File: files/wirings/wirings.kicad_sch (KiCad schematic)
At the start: 6 parts

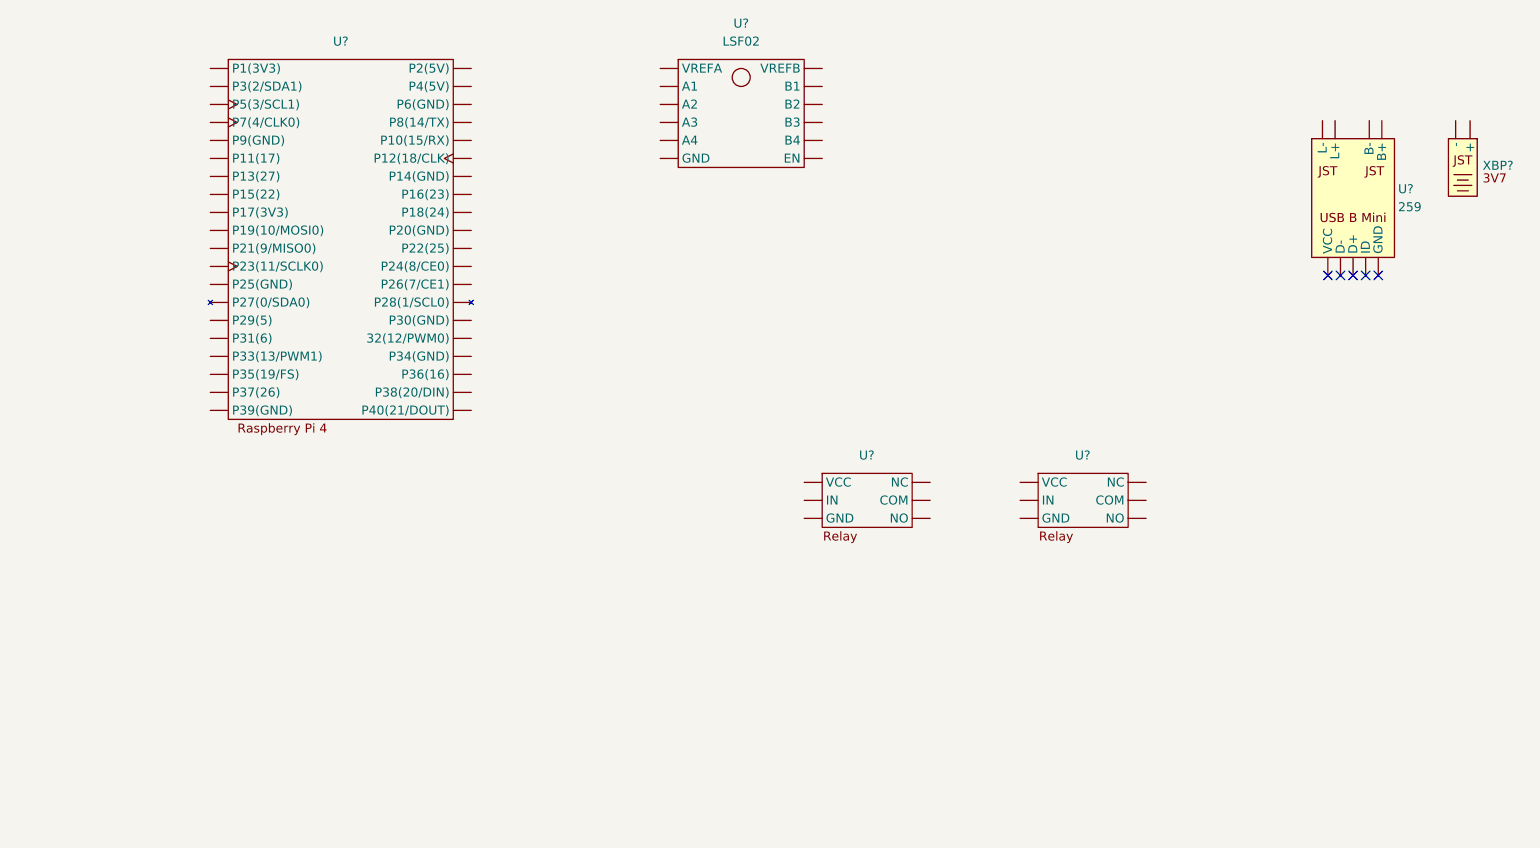
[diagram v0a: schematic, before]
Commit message: 14062023
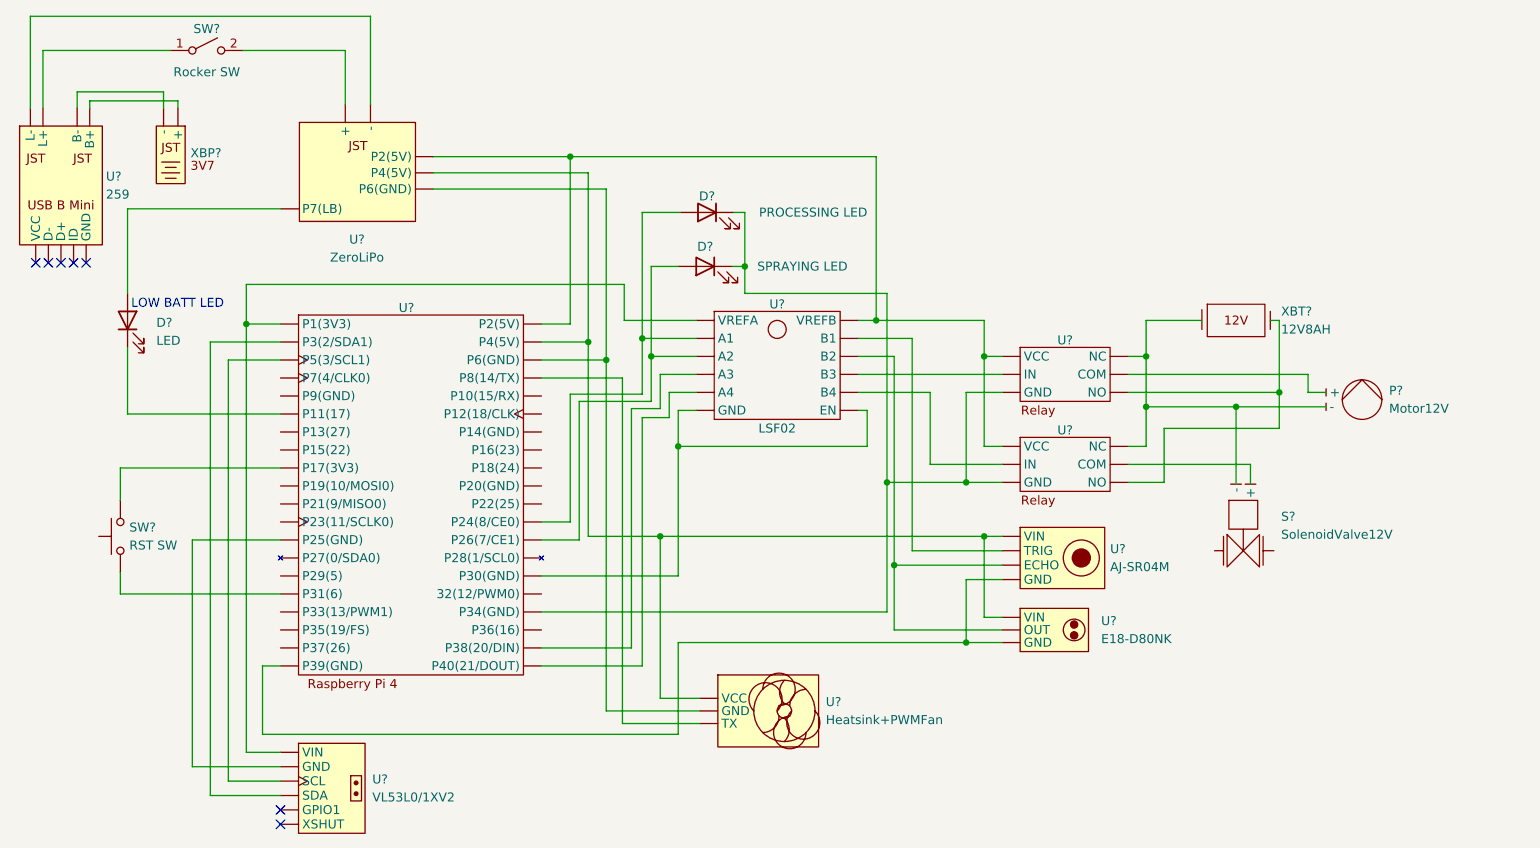
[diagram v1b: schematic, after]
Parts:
- added D?: PROCESSING LED, symbol Device:LED
- added D?: SPRAYING LED, symbol Device:LED
- added D?: LED, symbol Device:LED
- added P?: Motor12V, symbol Sensors and Others:Motor12V
- added S?: SolenoidValve12V, symbol Sensors and Others:SolenoidValve12V
- added SW?: Rocker SW, symbol Switch:SW_SPST
- added SW?: RST SW, symbol Switch:SW_Push
- added U?: VL53L0/1XV2, symbol Sensors and Others:VL53L0/1XV2
- added U?: Heatsink+PWMFan, symbol Sensors and Others:Heatsink+PWMFan
- added U?: E18-D80NK, symbol Sensors and Others:E18-D80NK
- added U?: ZeroLiPo, symbol Battery Power and Management:ZeroLiPo
- added U?: AJ-SR04M, symbol Sensors and Others:AJ-SR04M
- added XBT?: 12V8AH, symbol Battery Power and Management:12V8AH
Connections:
- net at U?. (VCC): now also P?. (-)
- net at U?. (VCC): now also U?. (VREFB)
- net at U?. (VCC): now also U?. (P7(LB))
- net at U?. (P9(GND)): now also D?.1 (K)
- net at XBP?. (-): now also U?. (VCC)
- net at U?. (VREFB): now also U?. (VIN)
- new net: P?. (-), S?. (-), U?. (VCC), U?. (VCC), XBT?. (-)
- new net: U?. (P7(LB)), U?. (P9(GND)), U?. (VCC), U?. (VCC), U?. (VREFB)
- new net: D?.1 (K), D?.1 (K), U?. (P9(GND)), U?. (VCC), U?. (VCC)
- new net: U?. (VCC), U?. (VCC), XBT?. (-)
- new net: U?. (VCC), U?. (VREFB)
- new net: S?. (-), U?. (VCC)
- new net: U?. (P9(GND)), U?. (XSHUT) (x3)
- new net: U?. (P9(GND)), U?. (VREFB), U?. (XSHUT)
- new net: U?. (P9(GND)), U?. (VCC)
- new net: U?. (P7(LB)), U?. (P9(GND)), U?. (VCC), U?. (VIN), U?. (VIN)
- new net: U?. (P7(LB)), U?. (P9(GND)), U?. (VCC)
- new net: U?. (VCC), XBP?. (-)
- new net: SW?.1 (A), U?. (VCC)
- new net: U?. (P9(GND)), U?. (VREFB) (x3)
- new net: D?.2 (A), U?. (P9(GND)), U?. (VREFB) (x2)
- new net: SW?.1, U?. (P9(GND))
- new net: SW?.2, U?. (P9(GND))
- new net: U?. (P9(GND)), U?. (VIN), U?. (VIN)
- new net: SW?.2 (B), U?. (P7(LB))
- new net: U?. (VIN), U?. (VIN), U?. (VREFB)
- new net: D?.2 (A), U?. (P7(LB))
- no-connect marks 5 -> 7
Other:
- note added: "LOW BATT LED"
- company: (none) -> There Goes Mangoes
- title: (none) -> Map of Wirings
- moved on the sheet: U?, XBP?

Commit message: 21062023
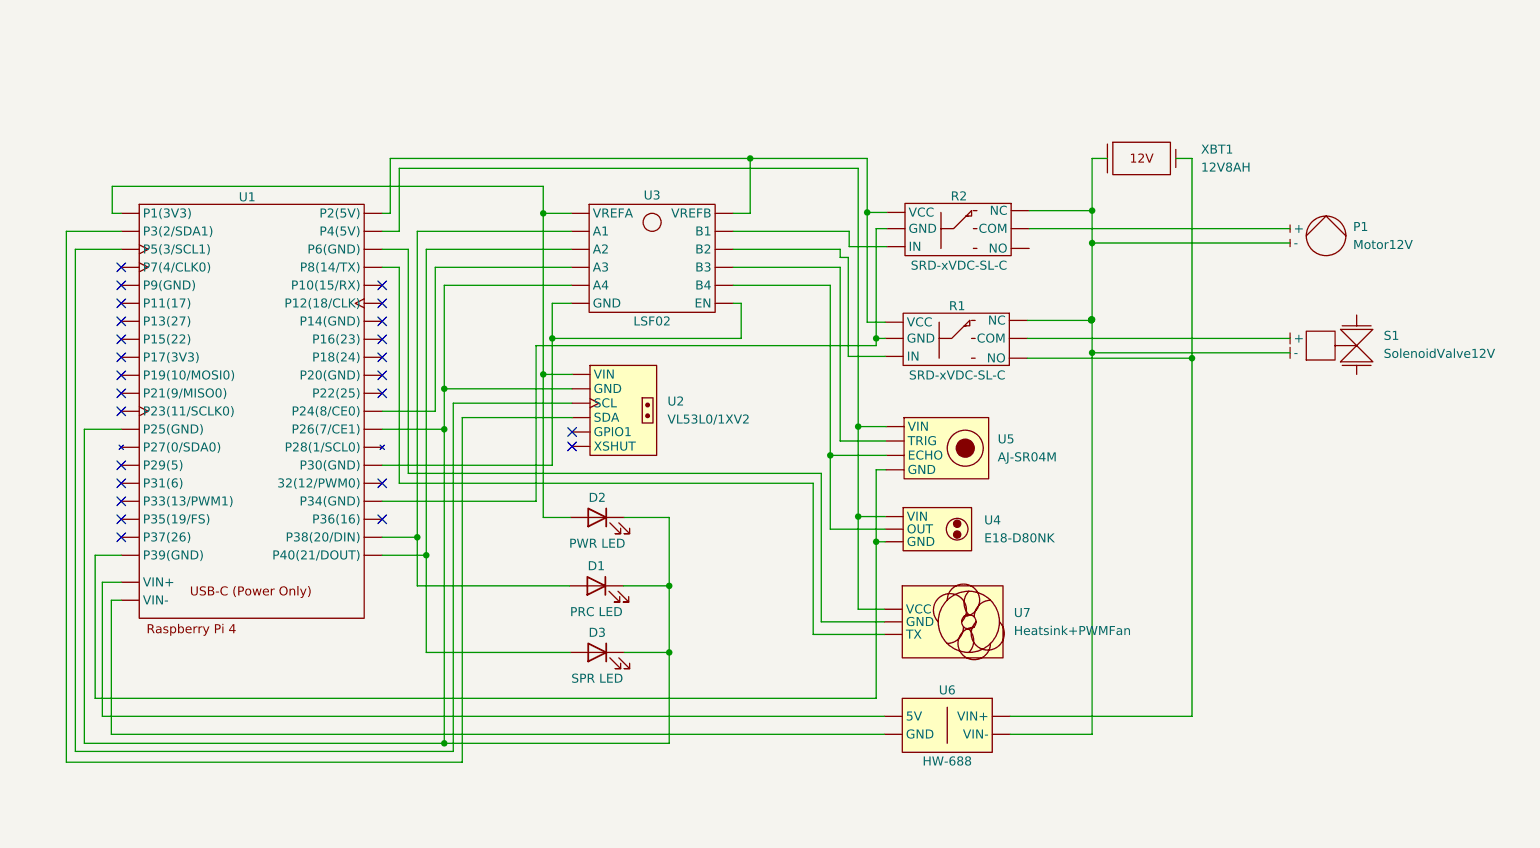
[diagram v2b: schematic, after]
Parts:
- removed D?: PROCESSING LED, symbol Device:LED
- removed D?: SPRAYING LED, symbol Device:LED
- removed D?: LED, symbol Device:LED
- removed P?: Motor12V, symbol Sensors and Others:Motor12V
- removed S?: SolenoidValve12V, symbol Sensors and Others:SolenoidValve12V
- removed SW?: Rocker SW, symbol Switch:SW_SPST
- removed SW?: RST SW, symbol Switch:SW_Push
- removed U? (x2): Songle_SRD-xxVDC-SL-C, symbol Relay:Songle_SRD-xxVDC-SL-C
- removed U?: VL53L0/1XV2, symbol Sensors and Others:VL53L0/1XV2
- removed U?: Heatsink+PWMFan, symbol Sensors and Others:Heatsink+PWMFan
- removed U?: 259, symbol Battery Power and Management:259
- removed U?: RPi4_Objective, symbol Raspberry Pi 4:RPi4_Objective
- removed U?: LSF02, symbol Multilevel Voltage Converter:LSF02
- removed U?: E18-D80NK, symbol Sensors and Others:E18-D80NK
- removed U?: ZeroLiPo, symbol Battery Power and Management:ZeroLiPo
- removed U?: AJ-SR04M, symbol Sensors and Others:AJ-SR04M
- removed XBP?: ICR18650-JST2P-PACK, symbol Battery Power and Management:ICR18650-JST2P-PACK
- removed XBT?: 12V8AH, symbol Battery Power and Management:12V8AH
- added D1: PRC LED, symbol Device:LED
- added D2: PWR LED, symbol Device:LED
- added D3: SPR LED, symbol Device:LED
- added P1: Motor12V, symbol Sensors and Others:Motor12V
- added R1, R2: SRD-xVDC-SL-C, symbol Sensors and Others:SRD-xVDC-SL-C
- added S1: SolenoidValve12V, symbol Sensors and Others:SolenoidValve12V
- added U1: RPi4_Objective, symbol Raspberry Pi 4:RPi4_Objective
- added U2: VL53L0/1XV2, symbol Sensors and Others:VL53L0/1XV2
- added U3: LSF02, symbol Multilevel Voltage Converter:LSF02
- added U4: E18-D80NK, symbol Sensors and Others:E18-D80NK
- added U5: AJ-SR04M, symbol Sensors and Others:AJ-SR04M
- added U6: HW-688, symbol Battery Power and Management:HW-688
- added U7: Heatsink+PWMFan, symbol Sensors and Others:Heatsink+PWMFan
- added XBT1: 12V8AH, symbol Battery Power and Management:12V8AH
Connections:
- new net: P1. (-), R2. (VCC)
- new net: P1. (-), R1. (VCC), R2. (VCC), S1. (-), U6. (VIN-), XBT1. (-)
- new net: D1.1 (K), D2.1 (K), D3.1 (K), U1. (VIN-), U2. (XSHUT), U3. (VREFB)
- new net: D2.2 (A), U1. (VIN-), U2. (XSHUT), U3. (VREFB)
- new net: R2. (VCC), U3. (VREFB)
- new net: R1. (VCC), R2. (VCC), U1. (VIN-), U3. (VREFB)
- new net: D3.2 (A), U1. (VIN-), U3. (VREFB)
- new net: U3. (VREFB), U5. (VIN)
- new net: U3. (VREFB), U4. (VIN), U5. (VIN)
- new net: D1.2 (A), U1. (VIN-), U3. (VREFB)
- new net: R1. (VCC), U3. (VREFB)
- new net: U1. (VIN-), U3. (VREFB) (x2)
- new net: R1. (VCC), R2. (VCC), U1. (VIN-)
- new net: R1. (VCC), U6. (VIN-), XBT1. (-)
- new net: U1. (VIN-), U4. (VIN), U5. (VIN), U7. (VCC)
- new net: U1. (VIN-), U4. (VIN), U5. (VIN)
- new net: R1. (VCC), S1. (-)
- new net: U1. (VIN-), U2. (XSHUT) (x2)
- new net: U1. (VIN-), U7. (VCC) (x2)
- new net: U1. (VIN-), U6. (VIN-) (x2)
- no-connect marks 7 -> 25
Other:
- note removed: "LOW BATT LED"
